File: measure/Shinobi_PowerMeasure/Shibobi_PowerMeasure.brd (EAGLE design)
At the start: 40.5 x 35 mm, 28 parts, among them M1 MCP73871

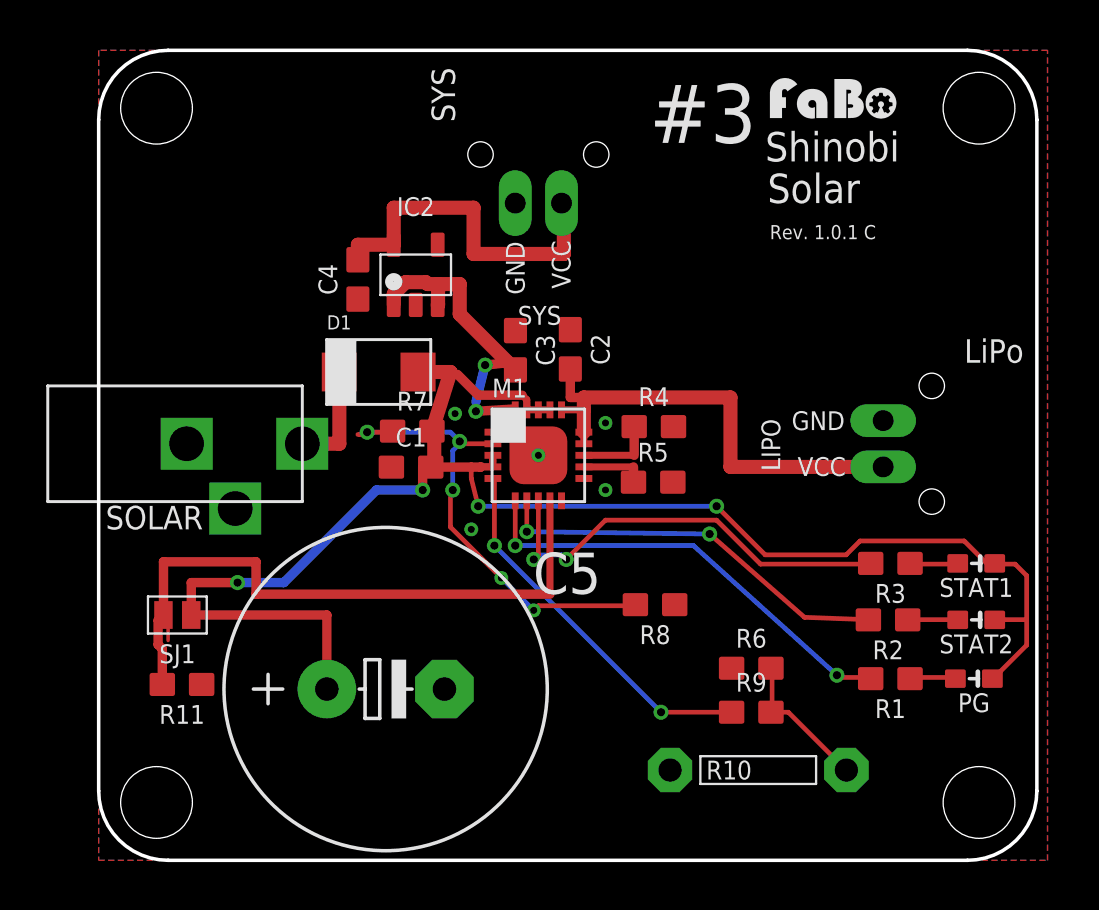
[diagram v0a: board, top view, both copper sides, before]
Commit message: Solar Add resistance constant,PowerMeasure
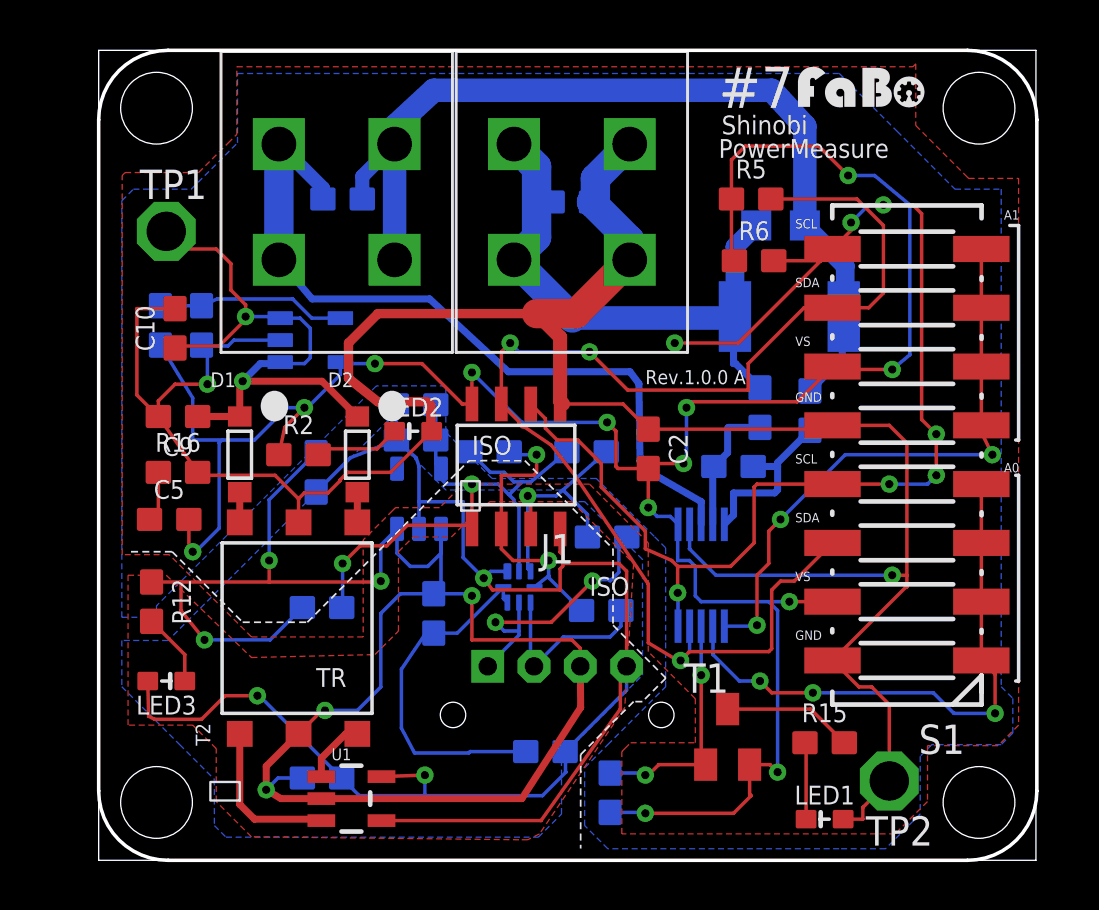
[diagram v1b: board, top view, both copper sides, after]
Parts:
- removed DC: 4UCON-DC, FaBo-Supply:4UCON-DC
- removed LIPO, SYS: FABO_BRICK_2PIN_SIDE, FaBo-Template:FABO_BRICK_2PIN_S02B−PASK-2_SILK
- removed M1: MCP73871, FaBo-Solar:QFN
- removed PG, STAT1, STAT2: (no value), FaBo-LED:0603
- removed SJ1: OPEN, FaBo-etc:SMD-JUMPER-2
- removed U$1: (no value), FaBo-Logo:LOGO_FABO_S
- added C10: 0.1uF, FaBo-Capacitor:0603
- added C6: 1uF, FaBo-Capacitor:0603
- added C7: NC, FaBo-Capacitor:0603
- added C8, C9: 10uF, FaBo-Capacitor:0603
- added D2: MBR0520L, FaBo:MBR0502L
- added IC1: 3.3V, FaBo-Supply:SOT-23-5
- added ISO: ISO1541, FaBo:ISO1541
- added J1: (no value), FaBo-Template:FABO_BRICK_I2C_S04B-PASK-2
- added LED1: RED, FaBo-LED:0603
- added LED2: GREEN, FaBo-LED:0603
- added LED3: BLUE, FaBo-LED:0603
- added R12: 1KΩ, FaBo-Resistors:0603
- added R13, R14: 4.7KΩ, FaBo-Resistors:0603
- added R15: 510Ω, FaBo-Resistors:0603
- added R16: 1Ω, FaBo-Resistors:0603
- added R17, R18, R19: NC, FaBo-Resistors:0603
- added S1: 219-08J, switch-dil:CTS-219-08J
- added SHUNT1: PMR10EZPFV2L00, FaBo:PMR10EZPFV2L00
- added SHUNT2: WSL2010R0250FEB, FaBo:WSL2010R0250FEB
- added T1: (no value), transistor:SC59-BEC
- added T2: 760390014, FaBo:760390014
- added TP1, TP2: TPPAD1-17, testpad:P1-17
- added U$3: ML-1400-S1, FaBo-Terminal:ML-1400-S1
- added U$5: (no value), FaBo-Template:FABO-SHINOBI
- added U$6: (no value), FaBo-Logo:LOGO_FABO_S
- added U$8: TPS76333, FaBo:TPS76333
- added U1: SN6501DBVR, TI:SOT-23-5
- added U2: TI-INA226, FaBo-Sensor:TI-INA226
- C1: value 10uf -> 0.1uF
- C2, C3: value 4.7uf -> 0.1uF
- C4: value 1uF -> 0.1uF
- C5: value NC -> 10uF; device rcl:E5-13 -> FaBo-Capacitor:0603
- D1: value DIODEDO-214AC -> MBR0520L; device FaBo-Diode:DO-214AC -> FaBo:MBR0502L
- IC2: device FaBo-Supply:SOT-23-5 -> FaBo-LevelTranslator:XQFN8
- R1: value 470 -> 4.7KΩ
- R10: value NTC Thermistor 10K -> 0Ω; device FaBo-Resistors:AXL-REGULAR -> FaBo-Resistors:0603
- R11: value 0 -> 0Ω
- R2: value 470 -> 1KΩ
- R3: value 470 -> NC
- R4: value 10K -> NC
- R5: value 10K -> 4.7KΩ
- R6: value 150K -> 4.7KΩ
- R7: value 270K -> 10Ω
- R8: value 100K -> 10Ω
- R9: value 240 -> 200KΩ
- U$2: value (none) -> ML-1400-S1; device FaBo-Template:FABO-SHINOBI -> FaBo-Terminal:ML-1400-S1
- moved R3 33.2 mm to (2.67, 23.1), flipped to the bottom, turned to 270 degrees
- moved R10 30.5 mm to (10.5, 28.6), flipped to the bottom, turned to 180 degrees
- moved U$2 30.3 mm to (10.3, 28.4)
- moved R11 26.8 mm to (20.4, 28.4), flipped to the bottom
- moved R2 26.5 mm to (8.64, 17.5), turned to 0 degrees
- moved C4 22.0 mm to (19.3, 4.70), flipped to the bottom, turned to 0 degrees
- moved R4 20.0 mm to (4.45, 23.1), flipped to the bottom, turned to 270 degrees
- moved R6 17.6 mm to (28.3, 25.9)
- moved R7 17.2 mm to (30.7, 19.4), flipped to the bottom, turned to 90 degrees
- moved R9 14.4 mm to (14.5, 10.7), flipped to the bottom, turned to 270 degrees
- moved IC2 14.2 mm to (18.2, 11.8), flipped to the bottom, turned to 270 degrees
- moved C1 13.9 mm to (27.4, 17.0), flipped to the bottom, turned to 180 degrees
- moved R1 13.1 mm to (22.1, 2.92), flipped to the bottom, turned to 270 degrees
- moved R5 12.9 mm to (28.2, 28.6)
- moved C5 11.9 mm to (3.05, 14.7)
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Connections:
- removed net LIPO_VCC: C2.2, LIPO.VCC, M1.P14, M1.P15, M1.P16
- removed net N$6: M1.P13, R4.1
- removed net SOLAR_VCC: C1.2, C5.+, D1.ANODE, M1.P17, M1.P18, M1.P19, M1.P3, M1.P4, PG.ANODE, R7.2, SJ1.1, STAT1.ANODE, STAT2.ANODE
- removed net SYS_VCC: C3.2, IC2.1, IC2.3, M1.P1, M1.P20
- removed net SYS_VCC_3V3: C4.2, IC2.5, SYS.VCC
- removed net TE: M1.P9, R11.2, SJ1.2
- removed net VPCC: M1.P2, R7.1, R8.2
- new net 3.3V: C2.2, C5.2, ISO.VCC2, R1.2, R2.1, R3.2, R5.1, R6.1, S1.11, S1.15, T1.E, U$8.OUT, U2.6
- new net A0: S1.1, S1.2, S1.3, S1.4, U2.2
- new net A1: S1.5, S1.6, S1.7, S1.8, U2.1
- new net GND_SECONDARY: C10.2, C2.1, C9.2, ISO.GND2, LED1.CATHODE, LED2.CATHODE, R11.2, R16.2, R4.2, S1.12, S1.16, T2.5, TP2.TP, U$3.RIGHT1, U$3.RIGHT2, U$8.GND, U2.7
- new net N$14: D1.P$2, T2.6
- new net N$15: D2.P$2, T2.4
- new net N$16: C10.1, C9.1, D1.P$1, D2.P$1, TP1.TP, U$8.EN, U$8.IN
- new net N$18: C4.2, IC2.7, IC2.8, R9.2
- new net N$19: C3.2, C8.2, IC1.1, IC1.3, J1.VCC, R12.1, R19.2, R9.1, T2.2, U1.2
- new net N$20: R3.1, R4.1, U$8.NC/FB
- new net N$21: C5.1, R16.1
- new net N$22: IC2.5, J1.SDA, R18.1
- new net N$23: IC2.3, ISO.SCL1, R13.1, R17.2
- new net N$7: LED1.ANODE, R15.1
- new net N$9: R15.2, T1.C
- new net SCL: ISO.SCL2, R6.2, S1.13, S1.9, U2.5
- new net SDA: ISO.SDA2, R5.2, S1.10, S1.14, U2.4
- new net VBUS: R10.1, U$2.LEFT1, U$2.LEFT2, U2.8
- new net VIN+: R10.2, R7.2, SHUNT1.P$2, SHUNT2.P$2, U$2.RIGHT1, U$2.RIGHT2
- new net VIN-: R11.1, R8.2, SHUNT1.P$1, SHUNT2.P$1, U$3.LEFT1, U$3.LEFT2
- net GND: now also C6.2, C7.2, C8.1, IC1.2, IC2.1, ISO.GND1, J1.GND, LED3.CATHODE, U1.4, U1.5; no longer C1.1, C2.1, C5.-, DC.GND1, IC2.2, LIPO.GND, M1.P$1, M1.P10, M1.P11, R10.1, R11.1, R4.2, R5.2, R6.1, R8.1, SYS.GND
- net N$1: now also C1.2, R7.1, U2.10; no longer PG.CATHODE, R1.1
- net N$10: now also LED3.ANODE, R12.2; no longer D1.CATHODE, DC.VCC
- net N$11: now also IC2.4, ISO.SDA1, R14.1, R18.2; no longer M1.P6, R1.2
- net N$12: now also IC2.6, J1.SCL, R17.1; no longer M1.P7, R2.2
- net N$13: now also C6.1, C7.1, IC1.5, IC2.2, ISO.VCC1, R13.2, R14.2, R19.1; no longer M1.P8, R3.2
- net N$2: now also C1.1, R8.1, U2.9; no longer R2.1, STAT2.CATHODE
- net N$3: now also T2.1, U1.3; no longer M1.P5, R9.1
- net N$4: now also T2.3, U1.1; no longer M1.P12, R5.1
- net N$5: now also R1.1, T1.B, U2.3; no longer R10.2, R6.2, R9.2
- net N$8: now also LED2.ANODE, R2.2; no longer R3.1, STAT1.CATHODE
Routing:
- net GND_SECONDARY: track 0.00 -> 109.4 mm, vias 0 -> 2
- net 3.3V: track 0.00 -> 104.5 mm, vias 0 -> 13
- net N$19: track 0.00 -> 75.8 mm, vias 0 -> 6
- net GND: track 0.00 -> 75.6 mm, vias 5 -> 3
- net SOLAR_VCC: track 71.5 -> 0.00 mm, vias 4 -> 0
- net SDA: track 0.00 -> 57.5 mm, vias 0 -> 3
- net SCL: track 0.00 -> 55.1 mm, vias 0 -> 7
- net VIN+: track 0.00 -> 40.6 mm
- net VBUS: track 0.00 -> 33.5 mm
- net TE: track 27.6 -> 0.00 mm
- net VIN-: track 0.00 -> 27.5 mm
- net N$16: track 0.00 -> 26.3 mm, vias 0 -> 2
- net A1: track 0.00 -> 25.7 mm, vias 0 -> 3
- net A0: track 0.00 -> 24.6 mm, vias 0 -> 3
- net VPCC: track 20.7 -> 0.00 mm, vias 5 -> 0
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- added copper zone on layer 1, net GND_SECONDARY
- added copper zone on layer 16, net GND_SECONDARY
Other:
- outline, holes or cut-outs redrawn
- board text added: "#7"
- board text added: "A0"
- board text added: "A1"
- board text added: "GND"
- board text added: "IN+"
- board text added: "IN-"
- board text added: "ISO"
- board text added: "PowerMeasure"
- board text added: "Rev.1.0.0 A"
- board text added: "S-PM01"
- board text added: "SCL"
- board text added: "SDA"
- board text added: "TR"
- board text added: "VBUS"
- board text added: "VS"
- board text removed: "#3"
- board text removed: "LiPo"
- board text removed: "Rev. 1.0.1 C"
- board text removed: "SOLAR"
- board text removed: "SYS"
- board text removed: "Solar"

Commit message: Dimention Delete
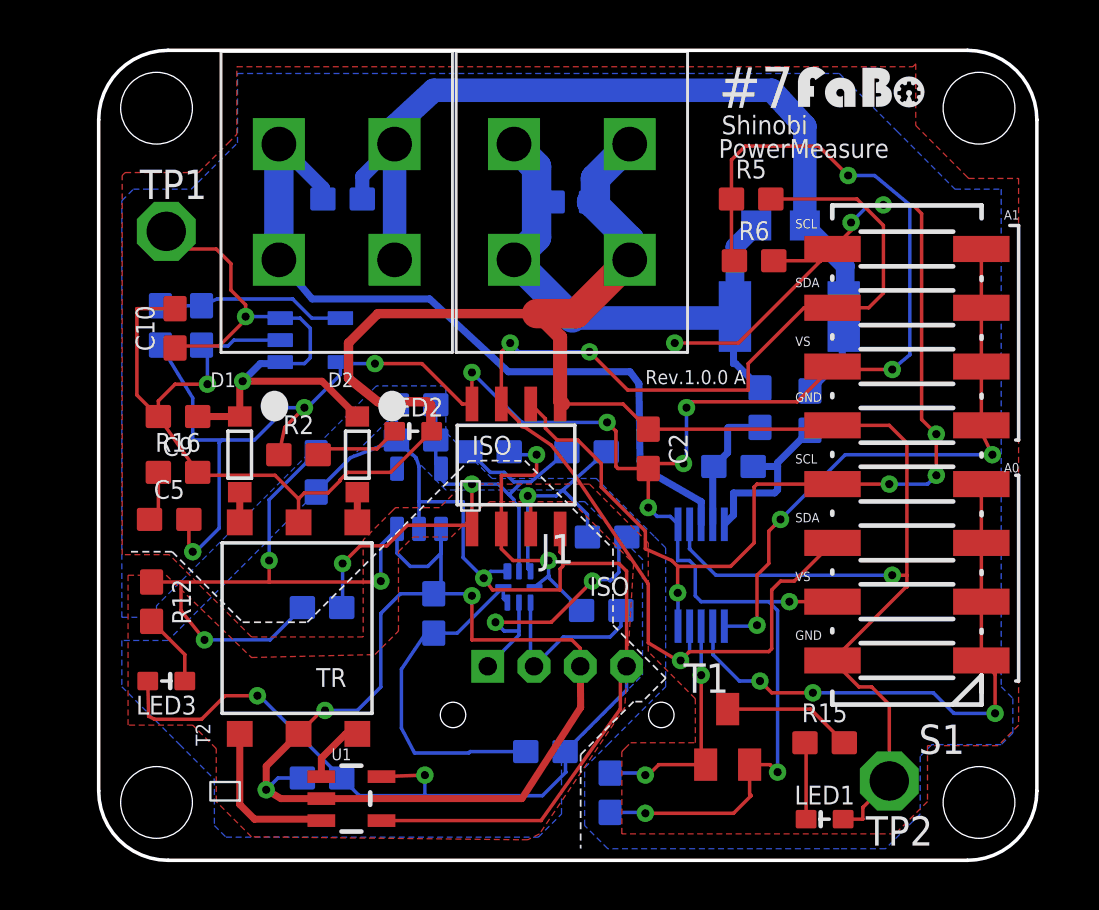
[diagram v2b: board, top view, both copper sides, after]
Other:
- outline, holes or cut-outs redrawn
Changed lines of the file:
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@@
 <?xml version="1.0" encoding="utf-8"?>
 <!DOCTYPE eagle SYSTEM "eagle.dtd">
-<eagle version="8.7.0">
+<eagle version="8.7.1">
 <drawing>
 <settings>
-<setting alwaysvectorfont="no"/>
+<setting alwaysvectorfont="yes"/>
 <setting verticaltext="up"/>
 </settings>
@@
 <board>
 <plain>
-<wire x1="0" y1="0" x2="40.5" y2="0" width="0" layer="20"/>
-<wire x1="40.5" y1="0" x2="40.5" y2="35" width="0" layer="20"/>
-<wire x1="40.5" y1="35" x2="0" y2="35" width="0" layer="20"/>
-<wire x1="0" y1="35" x2="0" y2="0" width="0" layer="20"/>
 <text x="26.789" y="30.353" size="0.8128" layer="21">PowerMeasure</text>
 <text x="26.789" y="32.512" size="1.778" layer="21">#7</text>
